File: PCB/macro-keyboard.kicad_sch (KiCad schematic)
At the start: 34 parts, among them P1 USB_C_Plug_USB2.0, SW1 DFU-mode, SW10 keySW, SW11 DFU-mode, SW2 RotaryEncoder, SW3 keySW, SW4 keySW, SW5 keySW, SW6 keySW, SW7 keySW, SW8 keySW, SW9 keySW, U1 CH552T

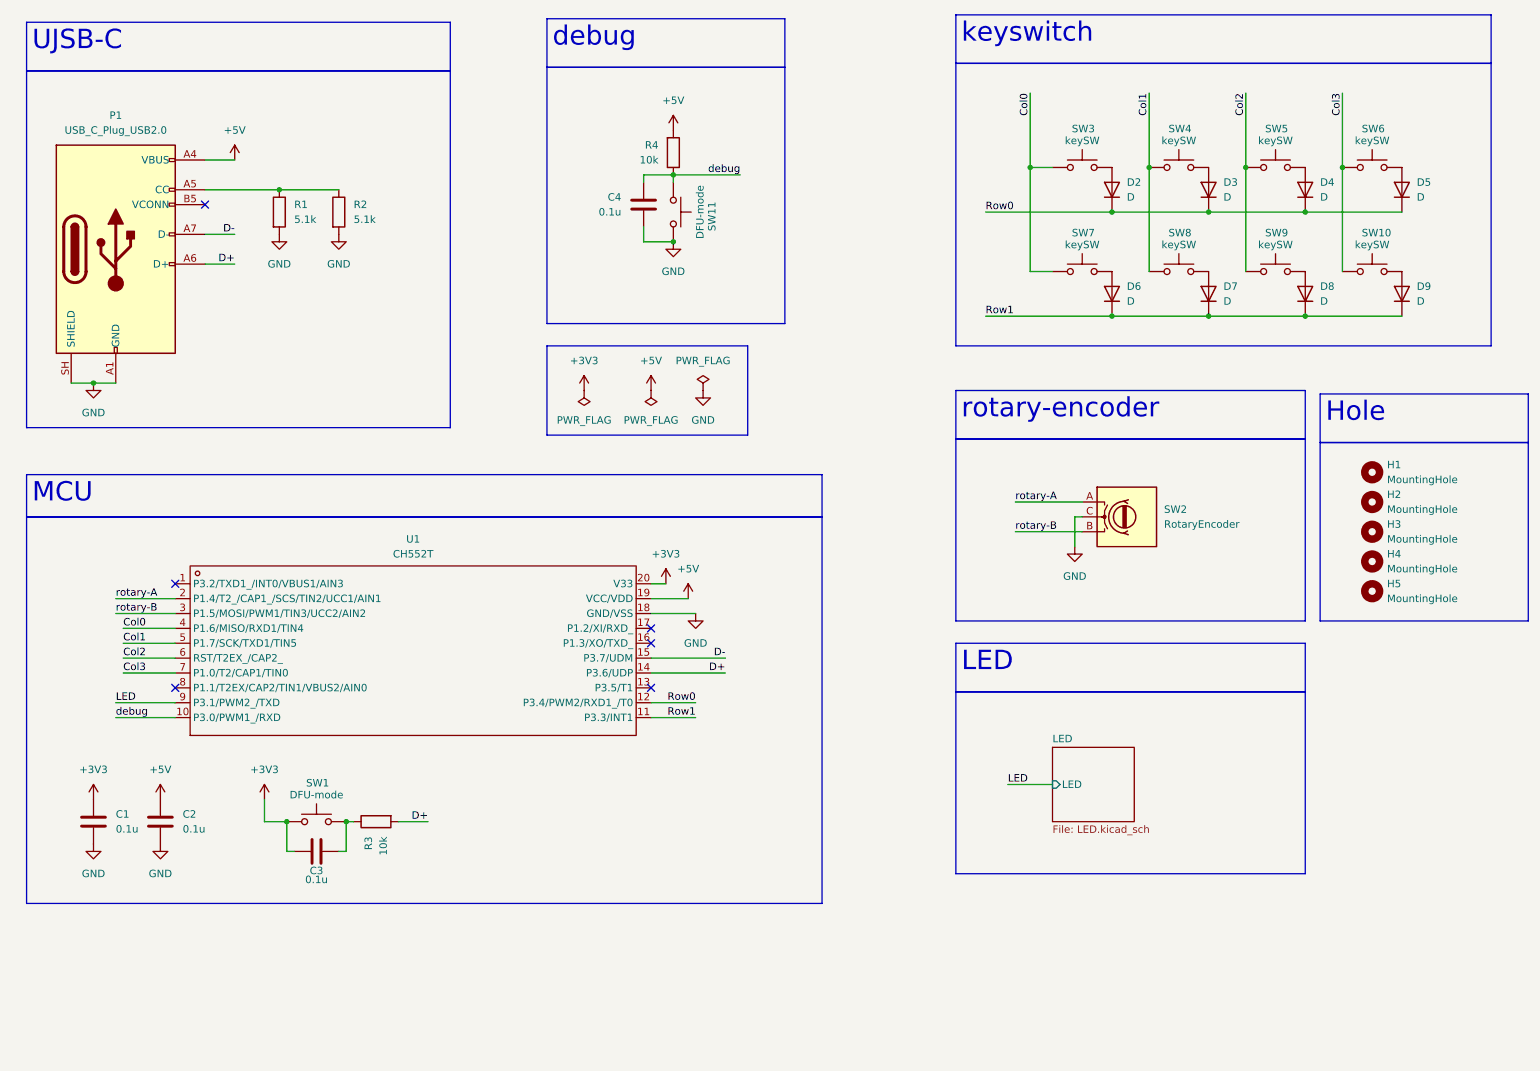
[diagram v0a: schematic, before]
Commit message: PCB作成（続き）
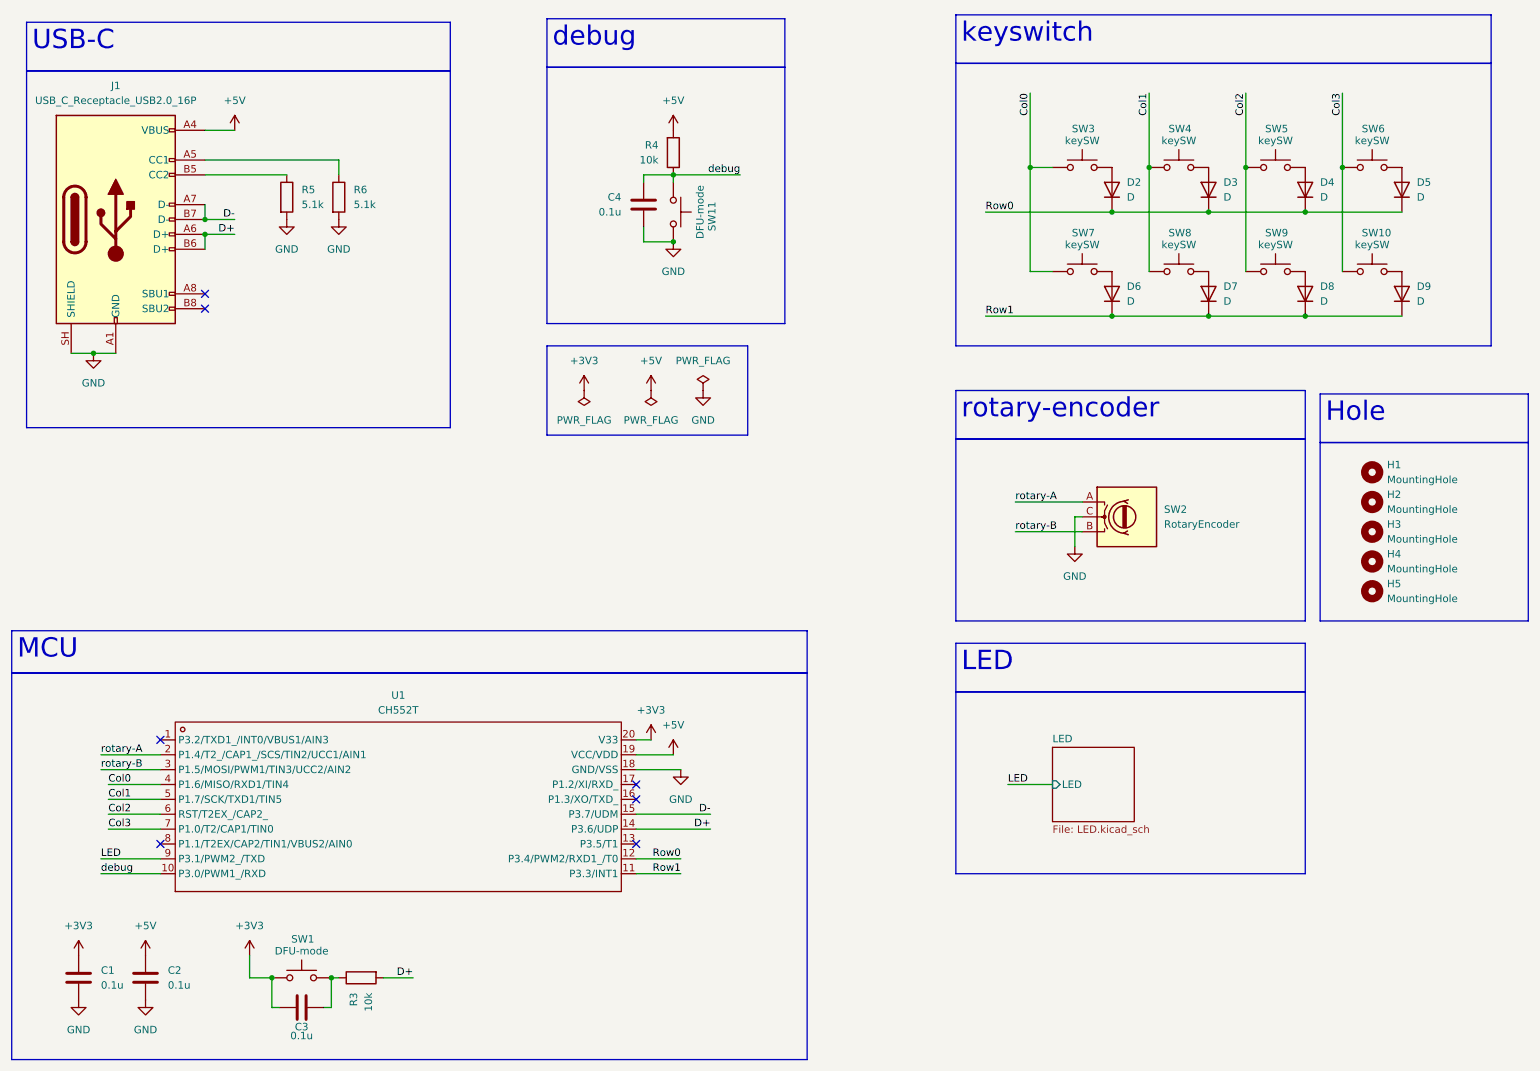
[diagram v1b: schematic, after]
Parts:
- removed P1: USB_C_Plug_USB2.0, Connector_USB:USB_C_Receptacle_GCT_USB4105-xx-A_16P_TopMnt_Horizontal, symbol Connector:USB_C_Plug_USB2.0
- removed R1, R2: 5.1k, Resistor_SMD:R_0603_1608Metric_Pad0.98x0.95mm_HandSolder, symbol Device:R
- added J1: USB_C_Receptacle_USB2.0_16P, Connector_USB:USB_C_Receptacle_GCT_USB4105-xx-A_16P_TopMnt_Horizontal, symbol Connector:USB_C_Receptacle_USB2.0_16P
- added R5, R6: 5.1k, Resistor_SMD:R_0603_1608Metric_Pad0.98x0.95mm_HandSolder, symbol Device:R
- SW2: footprint Rotary_Encoder:RotaryEncoder_Alps_EC12E-Switch_Vertical_H20mm -> Rotary_Encoder:RotaryEncoder_Alps_EC12E_Vertical_H20mm
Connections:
- net +5V: now also J1.A4 (VBUS), J1.A9 (VBUS), J1.B4 (VBUS), J1.B9 (VBUS)
- net D+: now also J1.A6 (D+), J1.B6 (D+)
- net D-: now also J1.A7 (D-), J1.B7 (D-)
- net GND: now also J1.A1 (GND), J1.A12 (GND), J1.B1 (GND), J1.B12 (GND), J1.SH (SHIELD), R5.2, R6.2
- new net: J1.A5 (CC1), R6.1
- new net: J1.B5 (CC2), R5.1
- no-connect marks 6 -> 7
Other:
- moved on the sheet: C1, C2, C3, R3, SW1, U1
